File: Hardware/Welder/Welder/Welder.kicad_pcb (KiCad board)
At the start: 2 copper layers, 165 x 95 mm, 70 parts, among them J1 Conn_01x08, J2 Screw_Terminal_01x03, J3 Screw_Terminal_01x02, J4 Screw_Terminal_01x02, Q1 Q_NMOS_GSD, Q2 Q_NMOS_GSD, SW1 SW_Push, SW2 SW_Push, SW3 SW_Push, U1 LM7805_TO220, U2 MOC3052M

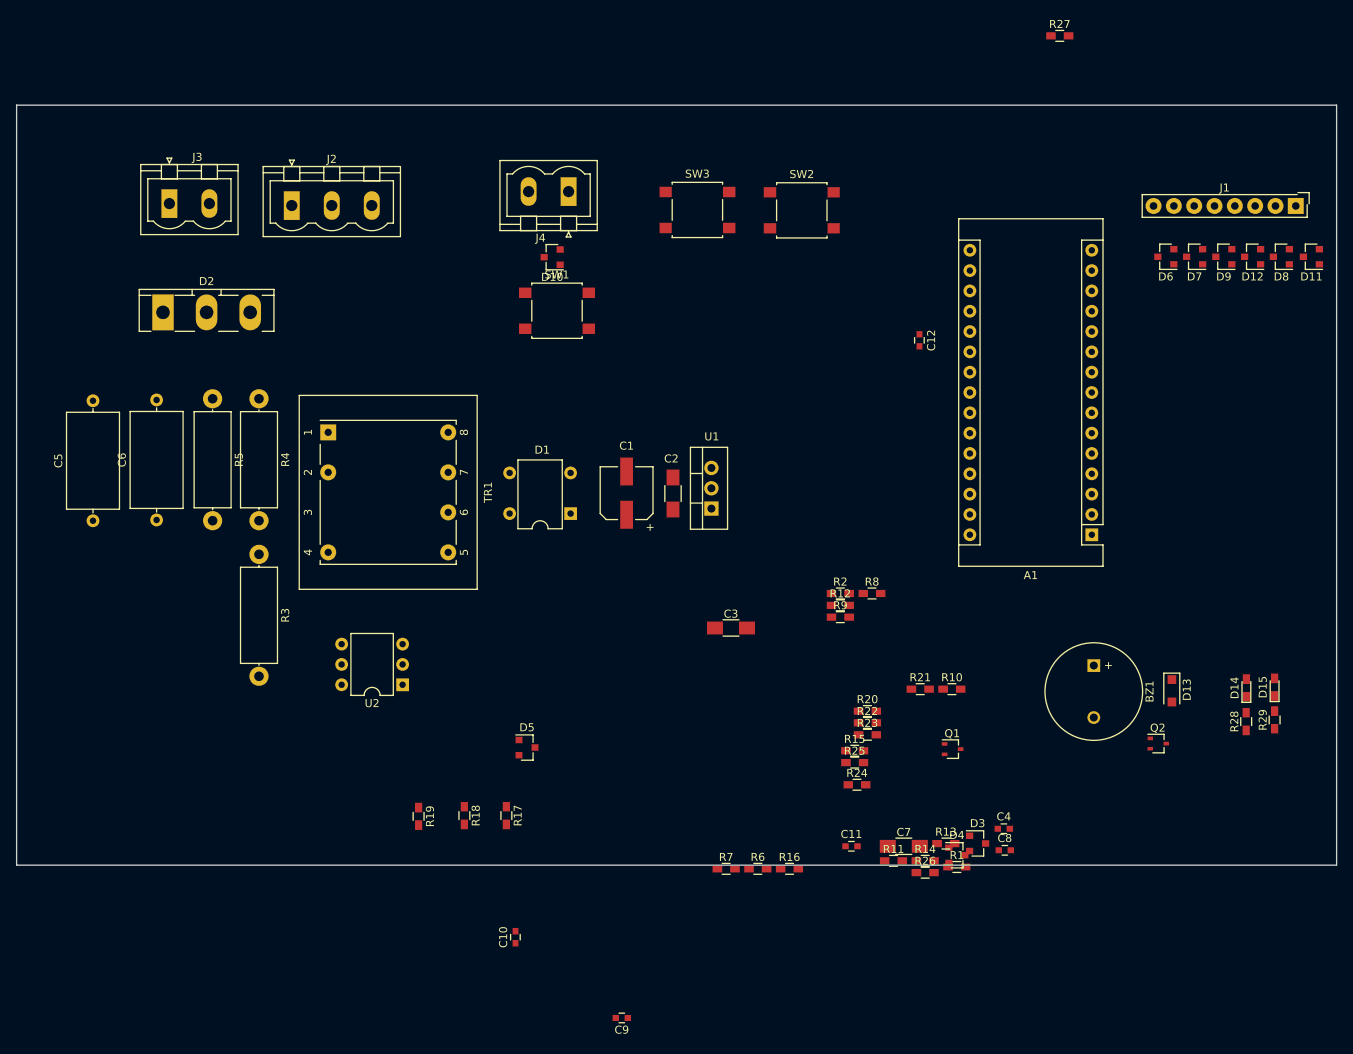
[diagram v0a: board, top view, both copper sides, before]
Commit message: Layout for Welder almost complete
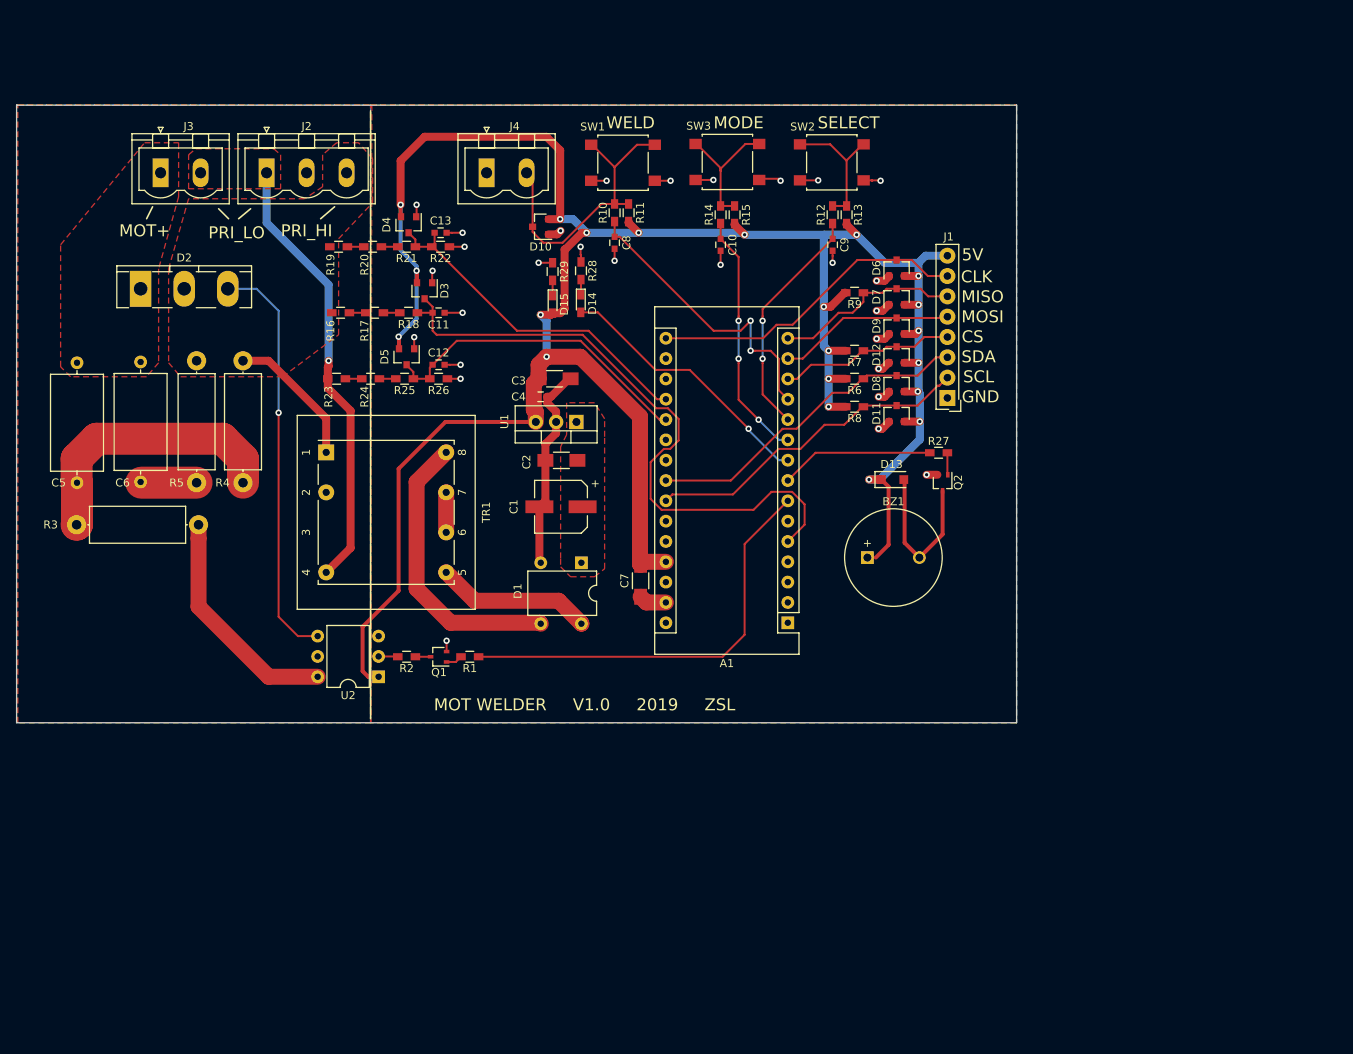
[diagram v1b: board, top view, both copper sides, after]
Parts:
- added C13: 10nF, Capacitors_SMD:C_0603, F.Cu at (98.0, 63.8)
- moved R29 106.2 mm to (112.0, 68.6), turned to 270 degrees
- moved D4 104.4 mm to (94.0, 62.8), turned to 270 degrees
- moved D15 102.2 mm to (112.0, 72.7), turned to 270 degrees
- moved R28 100.4 mm to (115.5, 68.5), turned to 270 degrees
- moved C9 100.2 mm to (147.0, 65.2), turned to 270 degrees
- moved D3 97.7 mm to (96.0, 71.0), turned to 270 degrees
- moved D14 96.1 mm to (115.5, 72.6), turned to 270 degrees
- moved C10 90.3 mm to (133.0, 65.2), turned to 270 degrees
- moved C8 90.3 mm to (119.8, 65.0), turned to 270 degrees
- moved R16 89.3 mm to (85.5, 73.8), turned to 180 degrees
- moved R11 87.5 mm to (121.5, 61.2), turned to 270 degrees
- moved R26 86.7 mm to (97.8, 82.0), turned to 180 degrees
- moved R20 84.8 mm to (89.5, 65.5), turned to 180 degrees
- moved R21 84.7 mm to (93.8, 65.5), turned to 180 degrees
- moved R14 84.7 mm to (133.0, 61.5), turned to 90 degrees
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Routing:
- net +5V: track 0.00 -> 322.4 mm, vias 0 -> 21
- net ZERO_CROSS: track 0.00 -> 80.4 mm
- net GND: track 0.00 -> 80.4 mm, vias 0 -> 28
- net PRI_LO: track 0.00 -> 55.6 mm, vias 0 -> 1
- net MOT_EN: track 0.00 -> 53.4 mm
- net Net-(D2-Pad3): track 0.00 -> 51.6 mm, vias 0 -> 1
- net PRIMARY_A_AI: track 0.00 -> 43.2 mm
- net SDA: track 0.00 -> 41.6 mm
- net SCL: track 0.00 -> 41.6 mm
- net PRIMARY_B_AI: track 0.00 -> 40.5 mm
- net CLK: track 0.00 -> 40.1 mm
- net WELD_BUTTON: track 0.00 -> 37.5 mm, vias 0 -> 2
- net WELD_BUTTON_OUT: track 0.00 -> 37.1 mm
- net Net-(D1-Pad3): track 0.00 -> 35.9 mm
- net Net-(C5-Pad1): track 0.00 -> 34.1 mm
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- added copper zone on B.Cu, net GND
- added copper zone on F.Cu, net GND
- added copper zone on F.Cu, net MOT_+
- added copper zone on F.Cu, net Net-(C1-Pad1)
- added copper zone on F.Cu, net PRI_HI
- added copper zone on F.Cu, net PRI_LO
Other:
- board size 165 x 95 mm -> 125 x 77.2 mm
- net class 5V added: clearance 0.2, trace_width 0.5, via_dia 0.8, via_drill 0.4
- board text added: "5V"
- board text added: "CLK"
- board text added: "CS"
- board text added: "GND"
- board text added: "MISO"
- board text added: "MODE"
- board text added: "MOSI"
- board text added: "MOT WELDER V1.0 2019 ZSL"
- board text added: "MOT+"
- board text added: "PRI_HI"
- board text added: "PRI_LO"
- board text added: "SCL"
- board text added: "SDA"
- board text added: "SELECT"
- board text added: "WELD"
